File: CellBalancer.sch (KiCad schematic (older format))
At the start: 12 parts, among them IC1 MAX923, Q1 IRF7455PBF

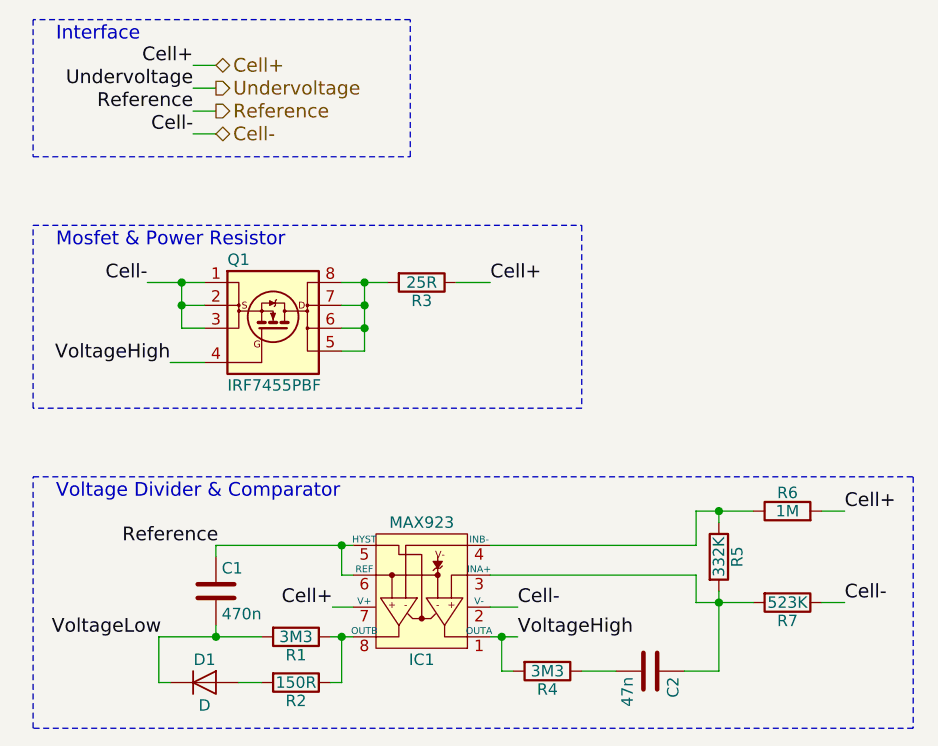
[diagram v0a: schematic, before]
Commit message: schematic done
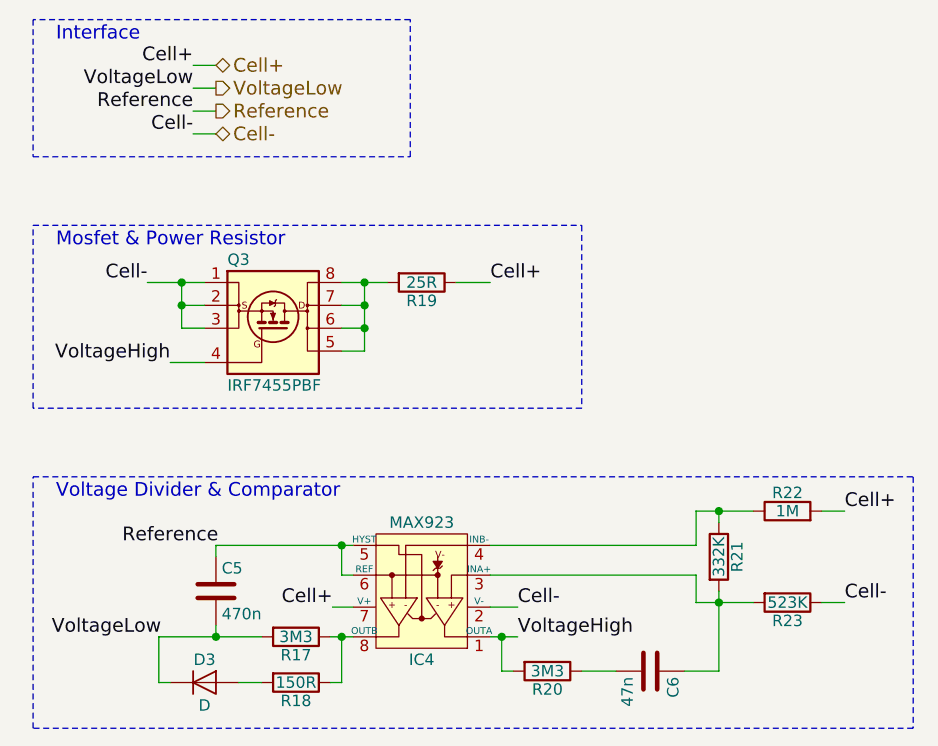
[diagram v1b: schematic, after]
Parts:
- renumbered IC1 to IC2, R1 to R3, R2 to R4, R3 to R5, R4 to R6, R5 to R7, R6 to R8, R7 to R9
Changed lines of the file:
@@
 $Descr A4 11693 8268
 encoding utf-8
-Sheet 2 4
+Sheet 4 4
 Title "Balancer"
 Date "2017-03-18"
@@
 Reference
 Text HLabel 1900 1100 2    60   Output ~ 0
-Undervoltage
+VoltageLow
 $Comp
 L IRF7455PBF Q1
@@
 AR Path="/58CDE720/58CDB997" Ref="Q2"  Part="1"
 AR Path="/58CDEEA6/58CDB997" Ref="Q3"  Part="1"
-F 0 "Q1" H 1950 2450 50  0000 L CNN
+F 0 "Q3" H 1950 2450 50  0000 L CNN
 F 1 "IRF7455PBF" H 1950 1900 50  0000 L CNN
 F 2 "Housings_SOIC:SOIC-8_3.9x4.9mm_Pitch1.27mm" H 2160 1740 50  0001 C CIN
@@
 $EndComp
 $Comp
-L R R3
+L R R5
 U 1 1 58CDB9A6
 P 2800 1950
-AR Path="/58CDDC72/58CDB9A6" Ref="R3"  Part="1"
-AR Path="/58CDE720/58CDB9A6" Ref="R10"  Part="1"
-AR Path="/58CDEEA6/58CDB9A6" Ref="R17"  Part="1"
-F 0 "R3" V 2880 1950 50  0000 C CNN
+AR Path="/58CDDC72/58CDB9A6" Ref="R5"  Part="1"
+AR Path="/58CDE720/58CDB9A6" Ref="R12"  Part="1"
+AR Path="/58CDEEA6/58CDB9A6" Ref="R19"  Part="1"
+F 0 "R19" V 2880 1950 50  0000 C CNN
 F 1 "25R" V 2800 1950 50  0000 C CNN
 F 2 "" V 2730 1950 50  0001 C CNN
@@
 $EndComp
 $Comp
-L R R6
+L R R8
 U 1 1 58CD80F2
 P 4400 2950
-AR Path="/58CDDC72/58CD80F2" Ref="R6"  Part="1"
-AR Path="/58CDE720/58CD80F2" Ref="R13"  Part="1"
-AR Path="/58CDEEA6/58CD80F2" Ref="R20"  Part="1"
-F 0 "R6" V 4480 2950 50  0000 C CNN
+AR Path="/58CDDC72/58CD80F2" Ref="R8"  Part="1"
+AR Path="/58CDE720/58CD80F2" Ref="R15"  Part="1"
+AR Path="/58CDEEA6/58CD80F2" Ref="R22"  Part="1"
+F 0 "R22" V 4480 2950 50  0000 C CNN
 F 1 "1M" V 4400 2950 50  0000 C CNN
 F 2 "" V 4330 2950 50  0001 C CNN
@@
 $EndComp
 $Comp
-L R R5
+L R R7
 U 1 1 58CD8143
 P 4100 3150
-AR Path="/58CDDC72/58CD8143" Ref="R5"  Part="1"
-AR Path="/58CDE720/58CD8143" Ref="R12"  Part="1"
-AR Path="/58CDEEA6/58CD8143" Ref="R19"  Part="1"
-F 0 "R5" V 4180 3150 50  0000 C CNN
+AR Path="/58CDDC72/58CD8143" Ref="R7"  Part="1"
+AR Path="/58CDE720/58CD8143" Ref="R14"  Part="1"
+AR Path="/58CDEEA6/58CD8143" Ref="R21"  Part="1"
+F 0 "R21" V 4180 3150 50  0000 C CNN
 F 1 "332K" V 4100 3150 50  0000 C CNN
 F 2 "" V 4030 3150 50  0001 C CNN
@@
 $EndComp
 $Comp
-L R R7
+L R R9
 U 1 1 58CD819C
 P 4400 3350
-AR Path="/58CDDC72/58CD819C" Ref="R7"  Part="1"
-AR Path="/58CDE720/58CD819C" Ref="R14"  Part="1"
-AR Path="/58CDEEA6/58CD819C" Ref="R21"  Part="1"
-F 0 "R7" V 4480 3350 50  0000 C CNN
+AR Path="/58CDDC72/58CD819C" Ref="R9"  Part="1"
+AR Path="/58CDE720/58CD819C" Ref="R16"  Part="1"
+AR Path="/58CDEEA6/58CD819C" Ref="R23"  Part="1"
+F 0 "R23" V 4480 3350 50  0000 C CNN
 F 1 "523K" V 4400 3350 50  0000 C CNN
 F 2 "" V 4330 3350 50  0001 C CNN
@@
 Cell+
 $Comp
-L MAX923 IC1
+L MAX923 IC2
 U 1 1 58CD8827
 P 2800 3300
-AR Path="/58CDDC72/58CD8827" Ref="IC1"  Part="1"
-AR Path="/58CDE720/58CD8827" Ref="IC2"  Part="1"
-AR Path="/58CDEEA6/58CD8827" Ref="IC3"  Part="1"
-F 0 "IC1" H 2800 3600 50  0000 C CNN
+AR Path="/58CDDC72/58CD8827" Ref="IC2"  Part="1"
+AR Path="/58CDE720/58CD8827" Ref="IC3"  Part="1"
+AR Path="/58CDEEA6/58CD8827" Ref="IC4"  Part="1"
+F 0 "IC4" H 2800 3600 50  0000 C CNN
 F 1 "MAX923" H 2800 3000 50  0000 C CNN
 F 2 "Housings_SOIC:SOIC-8_3.9x4.9mm_Pitch1.27mm" H 2810 2830 60  0001 C CIN
@@
 Cell-
 Text Label 1800 1100 2    60   ~ 0
-Undervoltage
+VoltageLow
 Text Label 1800 1200 2    60   ~ 0
 Reference
@@
 	2750 800  1100 800
 $Comp
-L R R4
+L R R6
 U 1 1 58CDBF0F
 P 3350 3650
-AR Path="/58CDDC72/58CDBF0F" Ref="R4"  Part="1"
-AR Path="/58CDE720/58CDBF0F" Ref="R11"  Part="1"
-AR Path="/58CDEEA6/58CDBF0F" Ref="R18"  Part="1"
-F 0 "R4" V 3430 3650 50  0000 C CNN
+AR Path="/58CDDC72/58CDBF0F" Ref="R6"  Part="1"
+AR Path="/58CDE720/58CDBF0F" Ref="R13"  Part="1"
+AR Path="/58CDEEA6/58CDBF0F" Ref="R20"  Part="1"
+F 0 "R20" V 3430 3650 50  0000 C CNN
 F 1 "3M3" V 3350 3650 50  0000 C CNN
 F 2 "" V 3280 3650 50  0001 C CNN
@@
 AR Path="/58CDE720/58CDBF54" Ref="C4"  Part="1"
 AR Path="/58CDEEA6/58CDBF54" Ref="C6"  Part="1"
-F 0 "C2" H 3825 3750 50  0000 L CNN
+F 0 "C6" H 3825 3750 50  0000 L CNN
 F 1 "47n" H 3825 3550 50  0000 L CNN
 F 2 "" H 3838 3500 50  0001 C CNN
@@
 Connection ~ 2450 3100
 $Comp
-L R R1
+L R R3
 U 1 1 58CDD170
 P 2250 3500
-AR Path="/58CDDC72/58CDD170" Ref="R1"  Part="1"
-AR Path="/58CDE720/58CDD170" Ref="R8"  Part="1"
-AR Path="/58CDEEA6/58CDD170" Ref="R15"  Part="1"
-F 0 "R1" V 2330 3500 50  0000 C CNN
+AR Path="/58CDDC72/58CDD170" Ref="R3"  Part="1"
+AR Path="/58CDE720/58CDD170" Ref="R10"  Part="1"
+AR Path="/58CDEEA6/58CDD170" Ref="R17"  Part="1"
+F 0 "R17" V 2330 3500 50  0000 C CNN
 F 1 "3M3" V 2250 3500 50  0000 C CNN
 F 2 "" V 2180 3500 50  0001 C CNN
@@
 $EndComp
 $Comp
-L R R2
+L R R4
 U 1 1 58CDD1EC
 P 2250 3700
-AR Path="/58CDDC72/58CDD1EC" Ref="R2"  Part="1"
-AR Path="/58CDE720/58CDD1EC" Ref="R9"  Part="1"
-AR Path="/58CDEEA6/58CDD1EC" Ref="R16"  Part="1"
-F 0 "R2" V 2330 3700 50  0000 C CNN
+AR Path="/58CDDC72/58CDD1EC" Ref="R4"  Part="1"
+AR Path="/58CDE720/58CDD1EC" Ref="R11"  Part="1"
+AR Path="/58CDEEA6/58CDD1EC" Ref="R18"  Part="1"
+F 0 "R18" V 2330 3700 50  0000 C CNN
 F 1 "150R" V 2250 3700 50  0000 C CNN
 F 2 "" V 2180 3700 50  0001 C CNN
@@
 AR Path="/58CDE720/58CDD221" Ref="D2"  Part="1"
 AR Path="/58CDEEA6/58CDD221" Ref="D3"  Part="1"
-F 0 "D1" H 1850 3800 50  0000 C CNN
+F 0 "D3" H 1850 3800 50  0000 C CNN
 F 1 "D" H 1850 3600 50  0000 C CNN
 F 2 "" H 1850 3700 50  0001 C CNN
@@
 AR Path="/58CDE720/58CDD43A" Ref="C3"  Part="1"
 AR Path="/58CDEEA6/58CDD43A" Ref="C5"  Part="1"
-F 0 "C1" H 1925 3400 50  0000 L CNN
+F 0 "C5" H 1925 3400 50  0000 L CNN
 F 1 "470n" H 1925 3200 50  0000 L CNN
 F 2 "" H 1938 3150 50  0001 C CNN
